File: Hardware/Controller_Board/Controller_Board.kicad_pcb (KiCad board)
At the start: 8 copper layers, 211 parts, among them J103 USB_C_USB2.0, Q1 DMN2400UFB-7, SW1 Reset, U1 TPS82084, U10 FT232H, U11 93LC56B, U12 USB2512B, U14 RJ45, U15 TPD4E02B04, U16 RJ45, U17 RJ45, U18 TPD4E02B04, U19 TPD4E02B04, U2 LT8645S, U20 TPD4E02B04, U21 TPD4E02B04, U22 RJ45, U23 TPD4E02B04, U24 TPD4E02B04, U25 RJ45, U26 TPD4E02B04, U27 TPD4E02B04, U28 RJ45, U29 TPD4E02B04, U3 TPS82084, U30 TPD4E02B04, U31 RJ45, U32 TPD4E02B04, U33 TPD4E02B04, U34 RJ45, U37 RJ45, U39 TPD4E02B04, U4 TPS82084, U5 XT30, U501 TPD4E02B04, U6 XC7A35T-CPG236, U7 IS25LP256D, U8 FT232H, U9 93LC56B, Y1 12MHz, Y2 12MHz, Y3 24MHz, Y301 12MHz

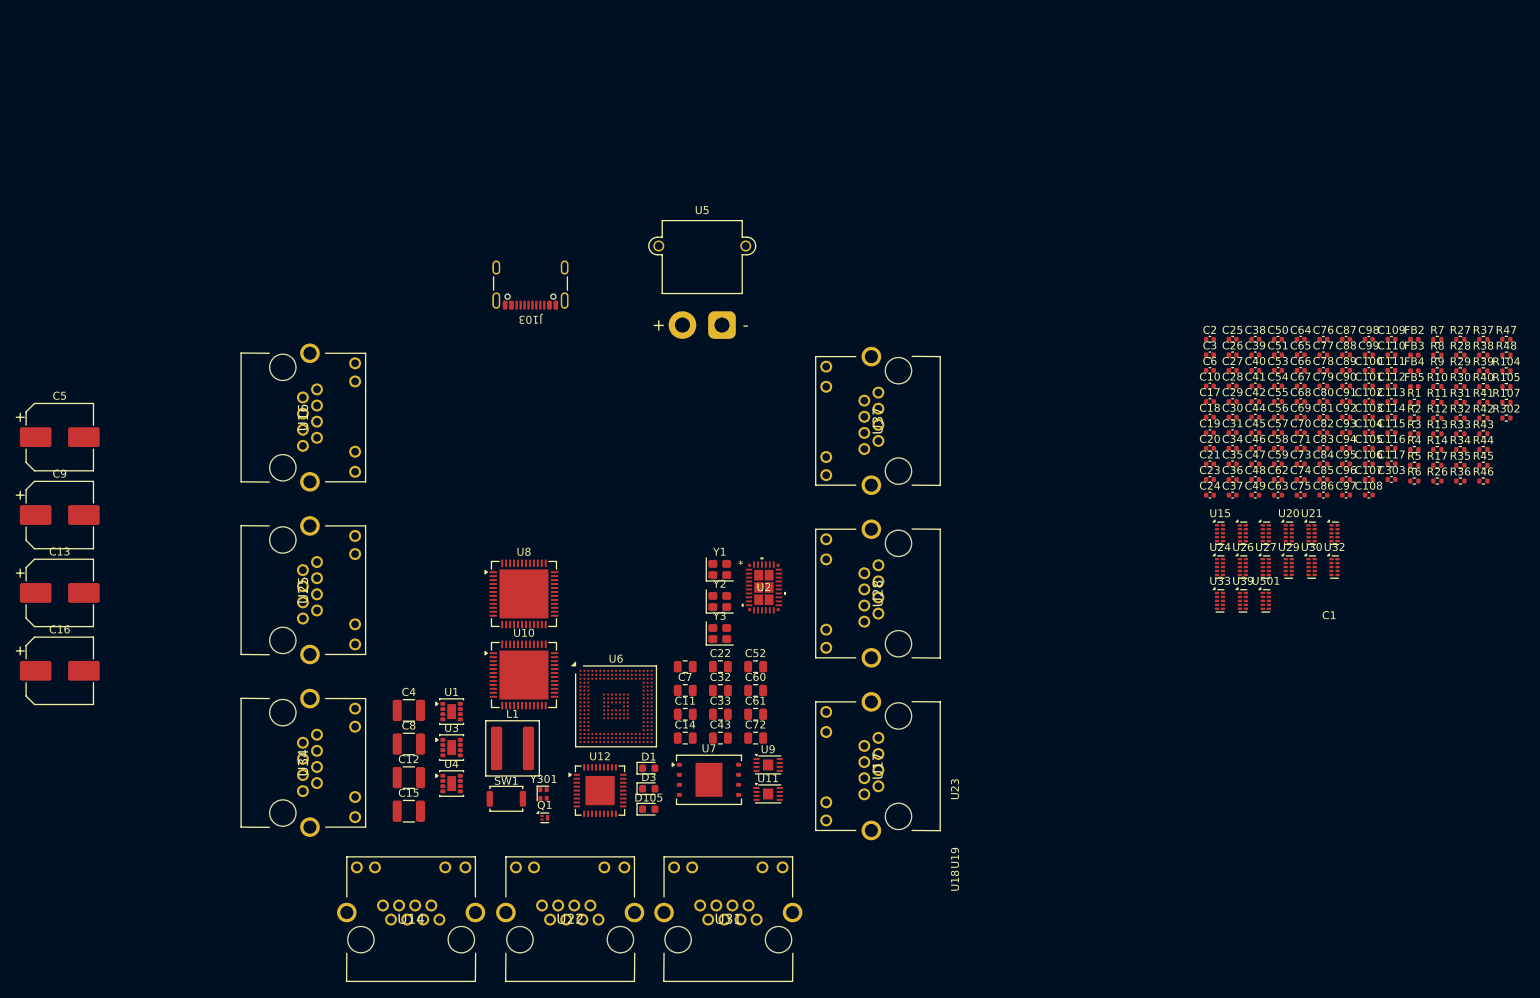
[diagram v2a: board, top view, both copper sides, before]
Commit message: Finished DRC check. Moving to schematic review
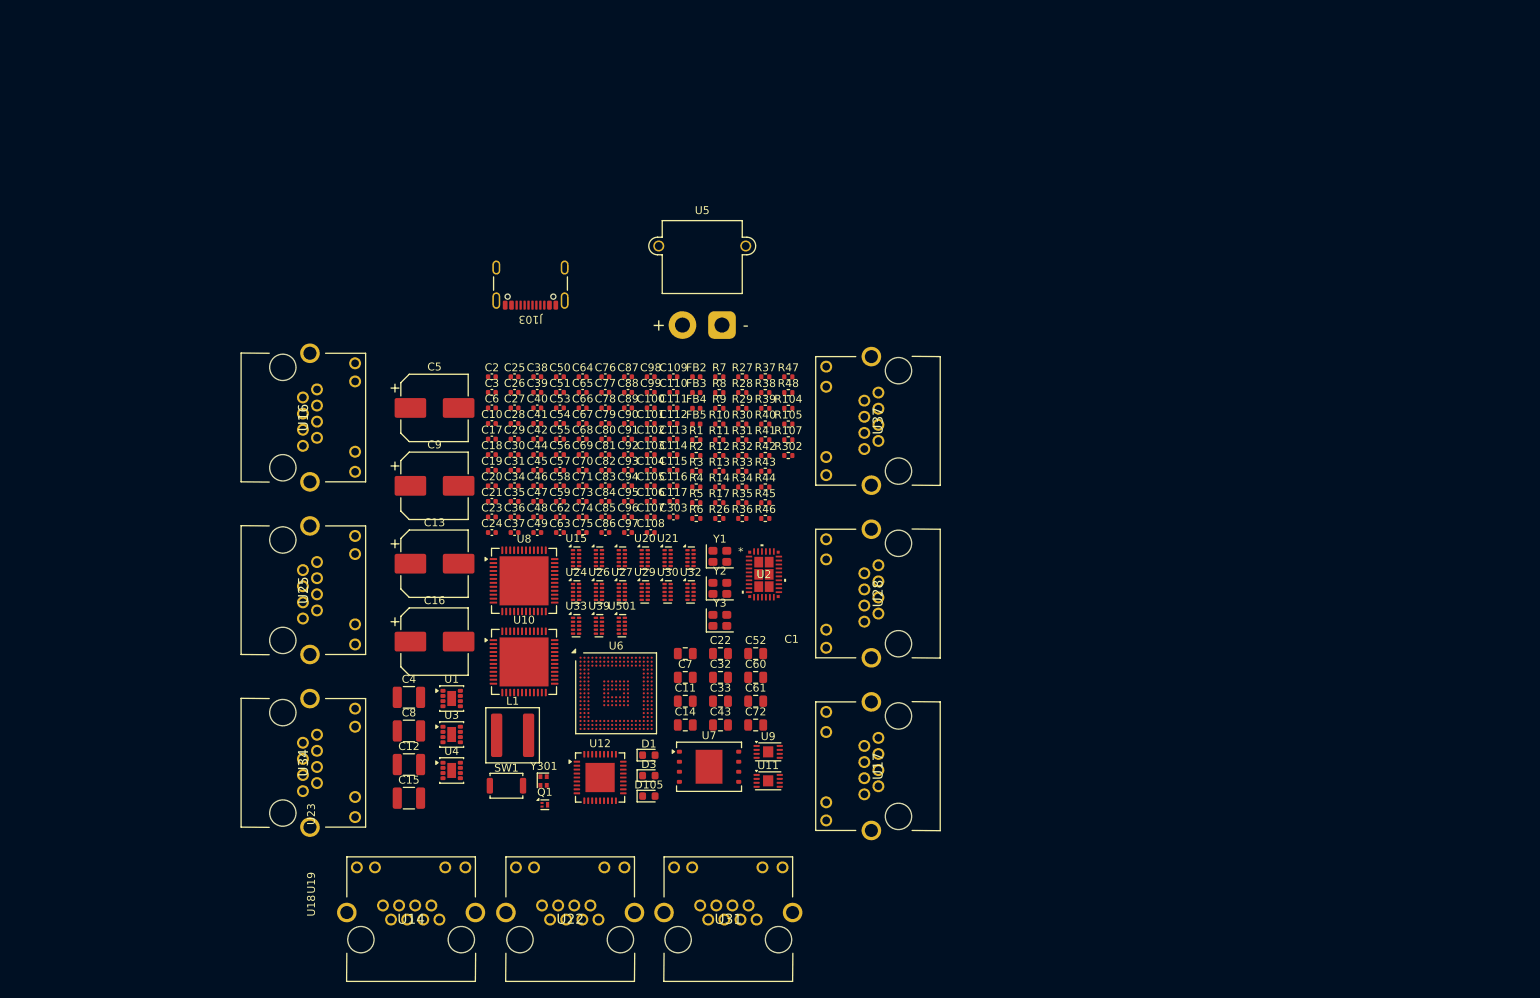
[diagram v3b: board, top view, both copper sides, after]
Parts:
- moved C50 90.9 mm to (121.7, 74.8)
- moved C51 90.9 mm to (121.7, 76.8)
- moved C53 90.9 mm to (121.7, 78.8)
- moved C54 90.9 mm to (121.7, 80.7)
- moved C55 90.9 mm to (121.7, 82.7)
- moved C56 90.9 mm to (121.7, 84.7)
- moved C57 90.9 mm to (121.7, 86.6)
- moved C58 90.9 mm to (121.7, 88.6)
- moved C59 90.9 mm to (121.7, 90.6)
- moved C62 90.9 mm to (121.7, 92.5)
- moved C63 90.9 mm to (121.7, 94.5)
- moved C10 90.9 mm to (113.1, 80.7)
- moved C100 90.9 mm to (133.2, 78.8)
- moved C101 90.9 mm to (133.2, 80.7)
- moved C102 90.9 mm to (133.2, 82.7)
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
